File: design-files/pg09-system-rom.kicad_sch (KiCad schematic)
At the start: 6 parts, among them U501 SST39SF040, U502 74AHC157, U503 74AHC157

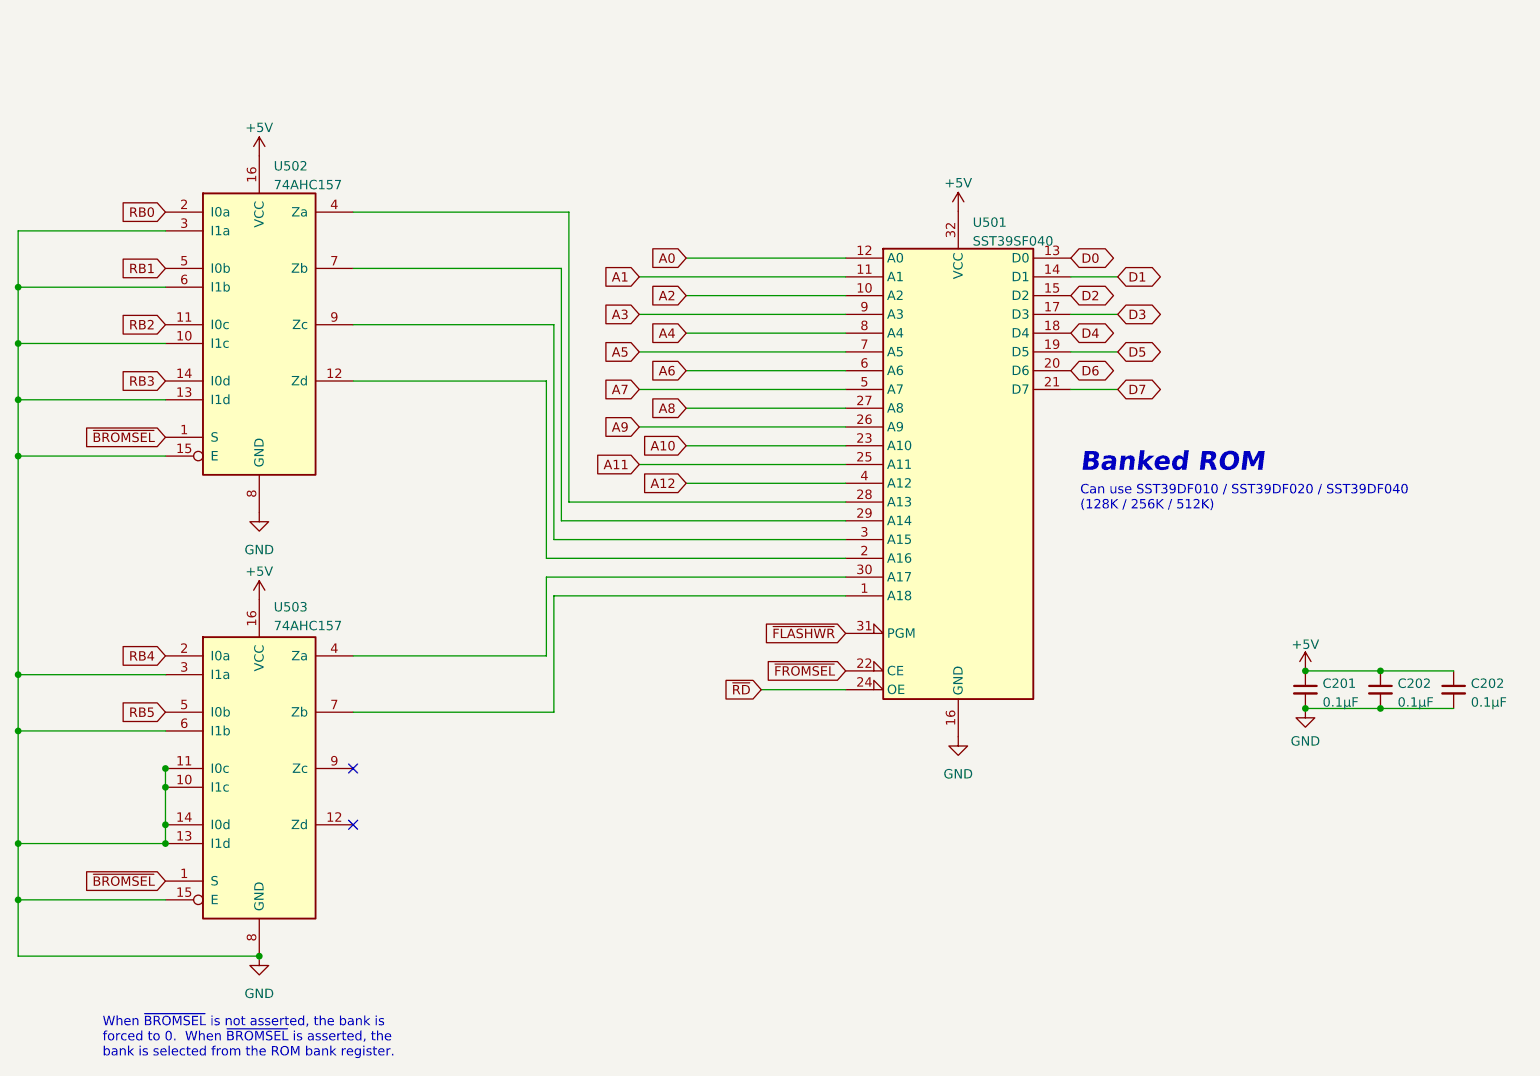
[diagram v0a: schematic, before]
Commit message: Simplify the fixed-vs-banked ROM selection logic.  Instead of using 2 '157 selectors, just use 2 '08 AND gate chips.  The bank signals are AND'd with /FROMSEL to force them to 0 when the fixed ROM is slected, and /FROMSEL and /BROMSEL are AND'd together to assert the flash ROM chip select whenever either one of them is asserted.
This reverts the /FROMSEL and /BROMSEL logic in ADDRDEC0 back to the
original equations.
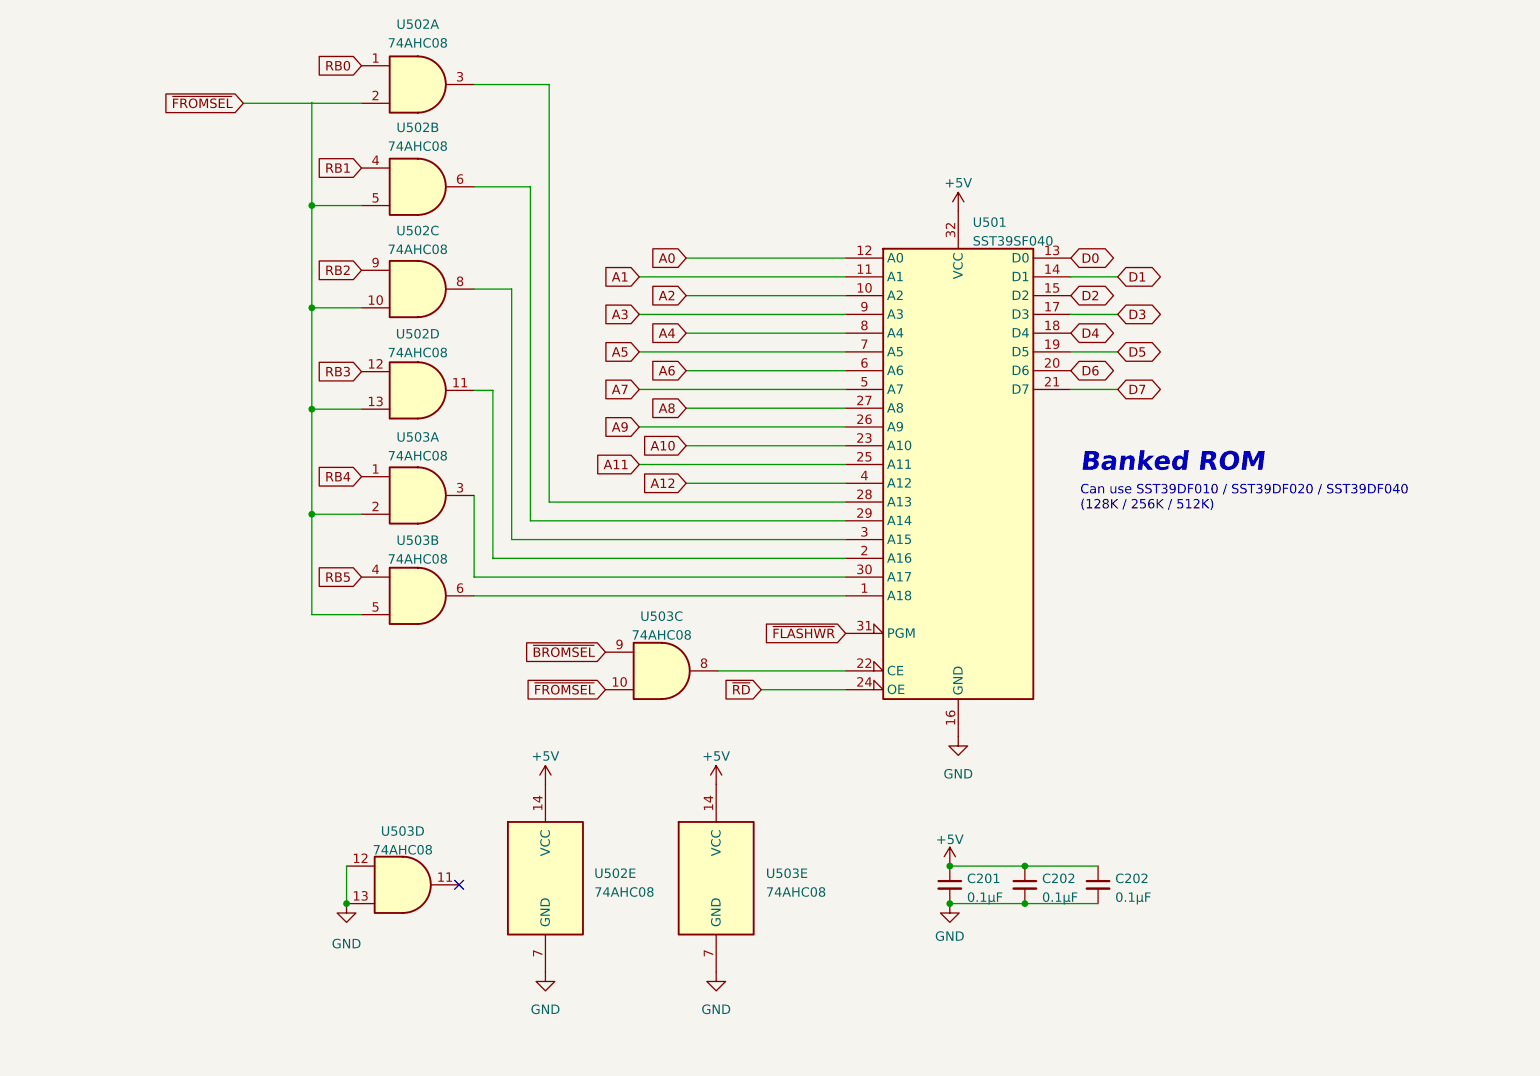
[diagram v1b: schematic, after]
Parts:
- removed U502, U503: 74AHC157, Package_DIP:DIP-16_W7.62mm_Socket, symbol 74xx:74LS157
- added U502, U503: 74AHC08, Package_DIP:DIP-14_W7.62mm_Socket, symbol 74xx:74LS08
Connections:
- net +5V: now also U502.14 (VCC), U503.14 (VCC)
- net GND: now also U502.7 (GND), U503.12, U503.13, U503.7 (GND)
- net RB0: now also U502.1
- net RB1: now also U502.4
- net RB2: now also U502.9
- net RB3: now also U502.12
- net RB4: now also U503.1
- net RB5: now also U503.4
- net ~{BROMSEL}: now also U503.9
- net ~{FROMSEL}: now also U502.2, U503.10; no longer U501.22 (CE)
- net at U501.30 (A17): now also U503.3
- net at U501.1 (A18): now also U503.6
- net at U501.2 (A16): now also U502.11
- net at U501.28 (A13): now also U502.3
- net at U501.29 (A14): now also U502.6
- net at U501.3 (A15): now also U502.8
- new net: U502.10, U502.13, U502.5, U503.2, U503.5
- new net: U501.22 (CE), U503.8
- no-connect marks 2 -> 1
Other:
- note removed: "When ~{BROMSEL} is not asserted, the bank is forced to 0. When ~{BROMSEL} is asserted, the bank is selected from the ROM bank register."
- moved on the sheet: C201, C202
